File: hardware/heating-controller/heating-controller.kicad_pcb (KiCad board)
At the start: 2 copper layers, 81.8 x 85.9 mm, 24 parts, among them J1 LilyGo T-Display S3, J2 Temperature_probes, J3 Power connector, K1 FINDER-32.21-x000, Q1 AO3400A, U1 H11AA1

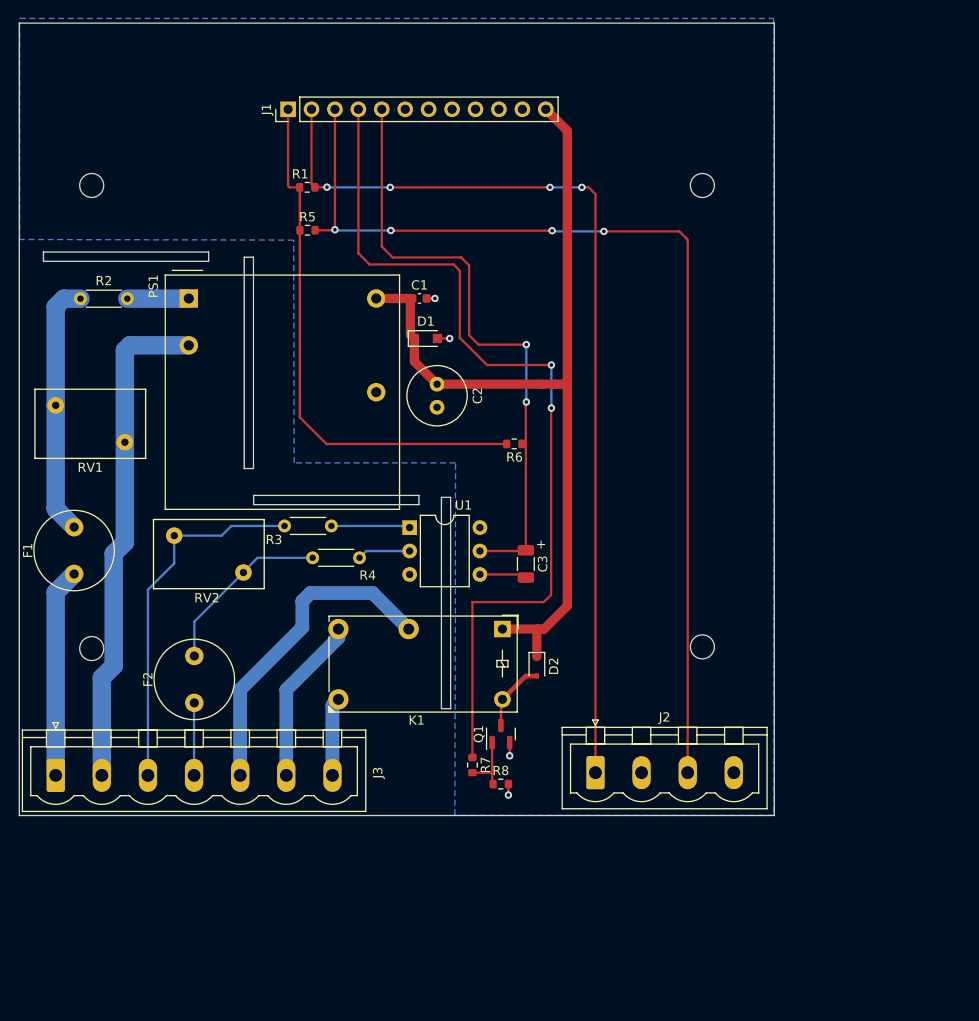
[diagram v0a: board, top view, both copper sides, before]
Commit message: WIP
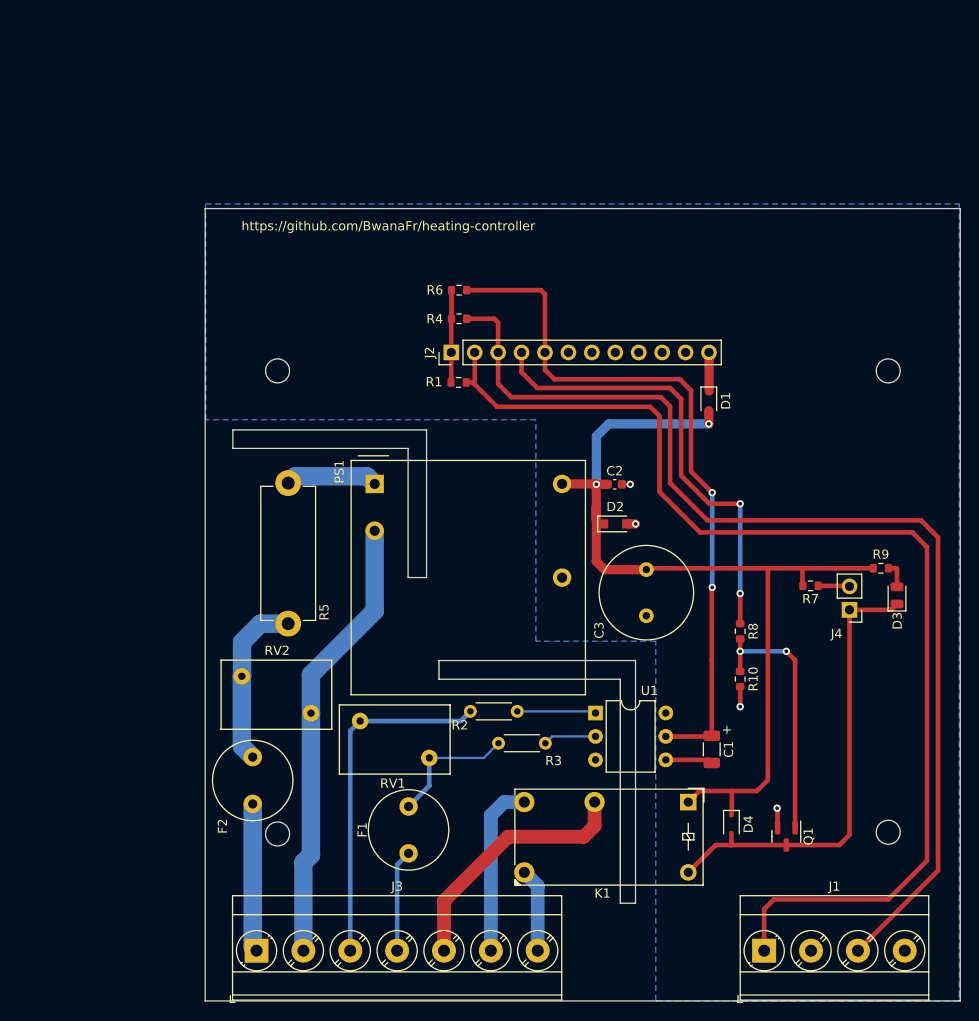
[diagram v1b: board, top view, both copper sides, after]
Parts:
- added D1: 1N4148WS, Diode_SMD:D_SOD-323, F.Cu at (74.8, 41.0)
- added D3: LED, LED_SMD:LED_0805_2012Metric, F.Cu at (95.2, 62.0)
- added J4: EXT_LED, Connector_PinHeader_2.54mm:PinHeader_1x02_P2.54mm_Vertical, F.Cu at (90.0, 63.6)
- added R7: 470, Resistor_SMD:R_0603_1608Metric, F.Cu at (85.8, 61.0)
- added R9: 470, Resistor_SMD:R_0603_1608Metric, F.Cu at (93.4, 59.1)
- C3: renamed from C2; footprint Capacitor_THT:C_Radial_D6.3mm_H7.0mm_P2.50mm -> Capacitor_THT:C_Radial_D10.0mm_H12.5mm_P5.00mm
- J1: renamed from J2; footprint Connector_Phoenix_MSTB:PhoenixContact_MSTBVA_2,5_4-G_1x04_P5.00mm_Vertical -> TerminalBlock_Phoenix:TerminalBlock_Phoenix_MKDS-3-4-5.08_1x04_P5.08mm_Horizontal
- J3: footprint Connector_Phoenix_MSTB:PhoenixContact_MSTBVA_2,5_7-G_1x07_P5.00mm_Vertical -> TerminalBlock_Phoenix:TerminalBlock_Phoenix_MKDS-3-7-5.08_1x07_P5.08mm_Horizontal
- R5: renamed from R2; footprint Resistor_THT:R_Axial_DIN0204_L3.6mm_D1.6mm_P5.08mm_Horizontal -> Resistor_THT:R_Axial_DIN0614_L14.3mm_D5.7mm_P15.24mm_Horizontal
- moved R5 41.8 mm to (29.1, 65.1), turned to 90 degrees
- moved RV2 35.6 mm to (24.1, 70.8)
- moved Q1 32.9 mm to (83.2, 88.2), turned to -90 degrees
- moved R8 32.4 mm to (78.2, 65.9)
- moved J2 31.7 mm to (46.8, 35.7)
- moved F2 31.6 mm to (25.3, 84.6)
- moved C3 30.3 mm to (68.0, 59.2)
- moved C2 29.2 mm to (64.5, 50.0)
- moved J3 28.9 mm to (25.7, 100.5)
- moved D2 28.7 mm to (64.6, 54.3)
- moved C1 28.5 mm to (75.1, 78.7)
- moved RV1 28.5 mm to (44.4, 79.7)
- moved PS1 28.5 mm to (36.0, 47.4)
- moved R2 28.5 mm to (48.9, 74.6)
- moved R3 28.5 mm to (52.0, 78.1)
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- renumbered C3 to C1, C1 to C2, D1 to D2, D2 to D4, F2 to F1, F1 to F2, J1 to J2, R8 to R10, R3 to R2, R4 to R3, R5 to R4, R7 to R8, RV2 to RV1, RV1 to RV2
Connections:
- J2 pad 12: +5V -> Net-(D1-Pad1)
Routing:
- net +3.3V: track 58.2 -> 10.0 mm
- net /RELAY_CMD: track 96.4 -> 49.6 mm
- net Net-(D3-Pad1): track 7.67 -> 50.2 mm
- net /EXT_TEMP: track 102.1 -> 123.8 mm, vias 4 -> 0
- net Net-(Q1-Pad1): track 6.73 -> 28.0 mm, vias 0 -> 2
- net /HP_ACTIVE: track 66.7 -> 77.0 mm
- net Net-(F2-Pad2): track 27.8 -> 18.8 mm
- net /REL_COM: track 35.2 -> 27.7 mm
- net +5V: track 94.3 -> 101.4 mm, vias 0 -> 2
- net /L: track 22.7 -> 16.1 mm
- net /LIMITER_TEMP: track 111.6 -> 118.1 mm, vias 4 -> 0
- net /N: track 54.3 -> 48.7 mm
- net Net-(F1-Pad2): track 19.5 -> 14.4 mm
- net Net-(D1-Pad1): track 0.00 -> 4.21 mm
- net Net-(J4-Pad2): track 0.00 -> 3.42 mm
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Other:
- outline, holes or cut-outs redrawn
- board text added: "https://github.com/BwanaFr/heating-controller"
